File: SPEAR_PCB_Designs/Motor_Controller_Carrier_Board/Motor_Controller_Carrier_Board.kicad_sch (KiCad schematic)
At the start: 14 parts, among them J1 Conn_01x02_Pin, J2 Conn_01x02_Pin, J3 Conn_01x02_Pin, J4 Conn_01x04_Pin, U1 AP63203WU

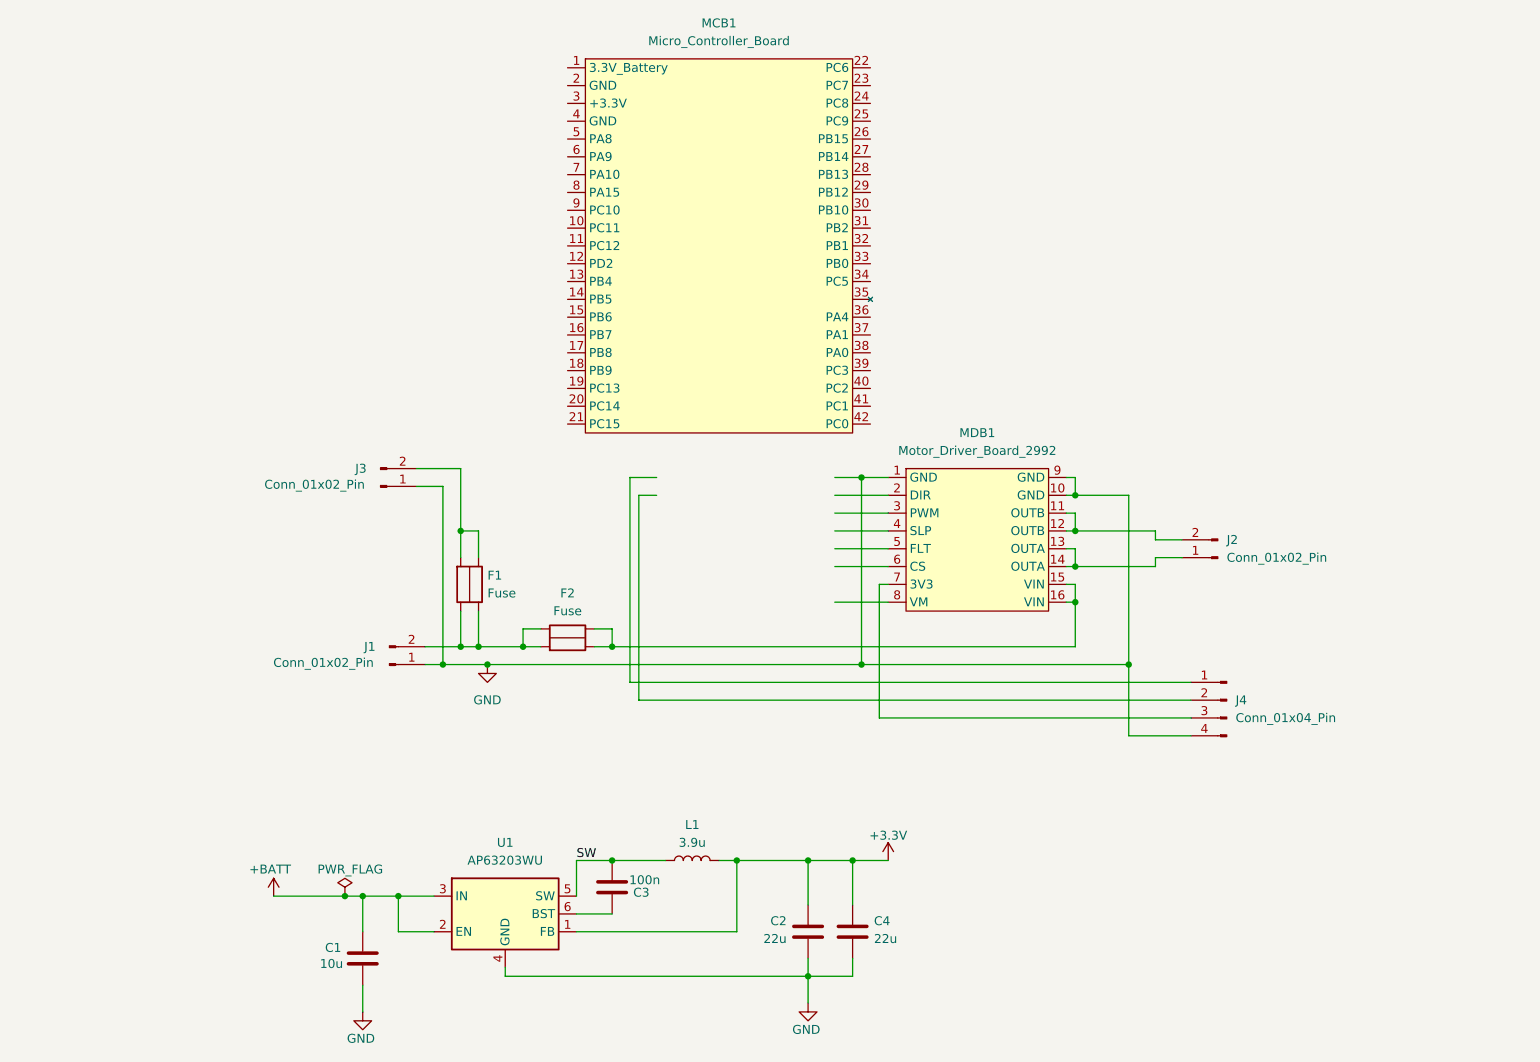
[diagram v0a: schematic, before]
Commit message: Finished schematic and general PCB layout for carrier board 2992
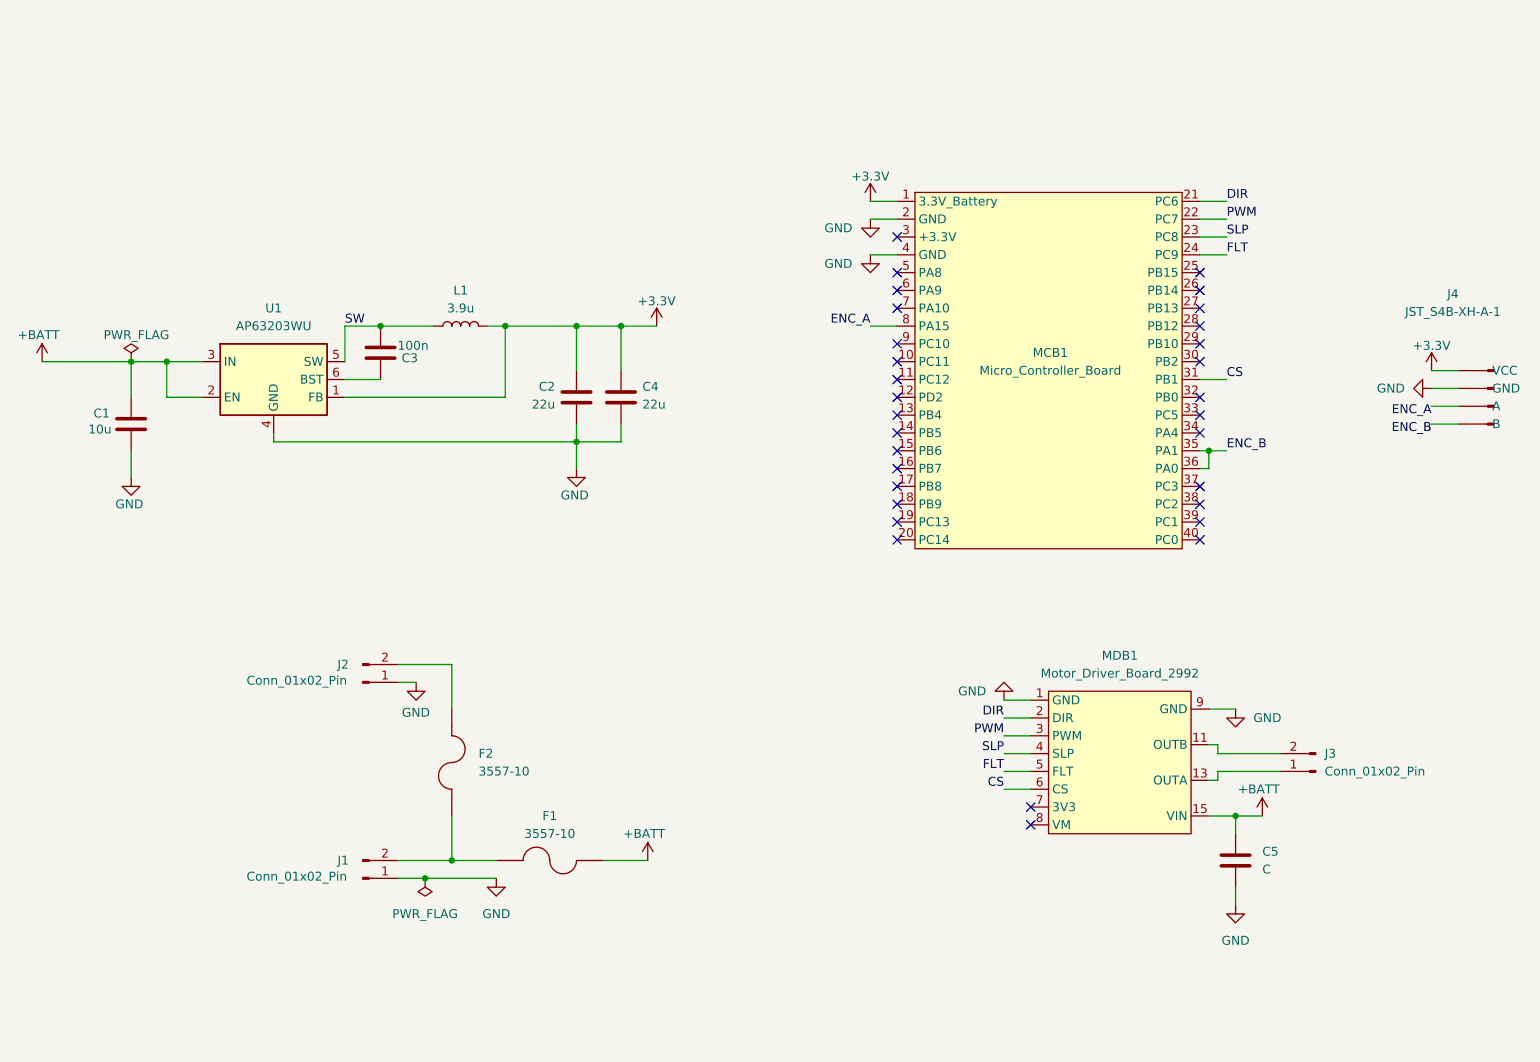
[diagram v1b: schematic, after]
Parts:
- removed F1, F2: Fuse, Motor_Controller_Carrier_Board:Fuse, symbol Motor_Controller_Carrier_Board:Fuse
- removed J4: Conn_01x04_Pin, Motor_Controller_Carrier_Board:JST_GH_BM04B-GHS-TBT_1x04-1MP_P1.25mm_Vertical, symbol Connector:Conn_01x04_Pin
- added C5: C, Motor_Controller_Carrier_Board:CAP_UBY_18X20_NCH, symbol Device:C
- added F1, F2: 3557-10, Motor_Controller_Carrier_Board:FUSE_3557-10, symbol Motor_Controller_Carrier_Board:3557-10
- added J4: JST_S4B-XH-A-1, Connector_JST:JST_XH_S4B-XH-A-1_1x04_P2.50mm_Horizontal, symbol Motor_Controller_Carrier_Board:JST_S4B-XH-A-1
- C1: footprint AP63202Footprints:CAP_FG20_TDK_C1 -> SPEAR_AP63203BuckConverter:CAP_FG20_TDK_C1
- C2, C4: footprint AP63202Footprints:CAP_FG22_TDK_C2_C4 -> SPEAR_AP63203BuckConverter:CAP_FG22_TDK_C2_C4
- L1: footprint AP63202Footprints:L_Wurth_WE-LHMI-1040_L1 -> SPEAR_AP63203BuckConverter:L_Wurth_WE-LHMI-1040_L1
- renumbered J3 to J2, J2 to J3
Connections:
- net +3.3V: now also MCB1.1 (3.3V_Battery), J4.4 (VCC)
- net +BATT: now also MDB1.15 (VIN), MDB1.16 (VIN), C5.1, F1.2_1, F1.2_2
- net GND: now also MCB1.2 (GND), MCB1.4 (GND), C5.2, J4.3 (GND)
- net DIR: now reaches MDB1.2 (DIR)
- net DIR: now also MCB1.21 (PC6)
- net PWM: now reaches MDB1.3 (PWM)
- net PWM: now also MCB1.22 (PC7)
- net SLP: now reaches MDB1.4 (SLP)
- net SLP: now also MCB1.23 (PC8)
- net FLT: now reaches MDB1.5 (FLT)
- net FLT: now also MCB1.24 (PC9)
- net CS: now reaches MDB1.6 (CS)
- net CS: now also MCB1.31 (PB1)
- net at J1.2 (Pin_2): now also F1.1_1, F1.1_2, F2.1_1, F2.1_2
- net at J2.2 (Pin_2): now also F2.2_1, F2.2_2
- net ENC_B: now reaches MCB1.35 (PA1)
- net ENC_B: now also MCB1.36 (PA0), J4.1 (B)
- net ENC_A: now reaches MCB1.8 (PA15)
- net ENC_A: now also J4.2 (A)
- no-connect marks 0 -> 31
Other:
- company: (none) -> SPEAR
- title: (none) -> Motor Controller Carrier Board
- moved on the sheet: C1, C2, C3, C4, J1, J2, J3, L1, U1
